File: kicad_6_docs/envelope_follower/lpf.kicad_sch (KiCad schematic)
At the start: 6 parts, among them U2 TL072

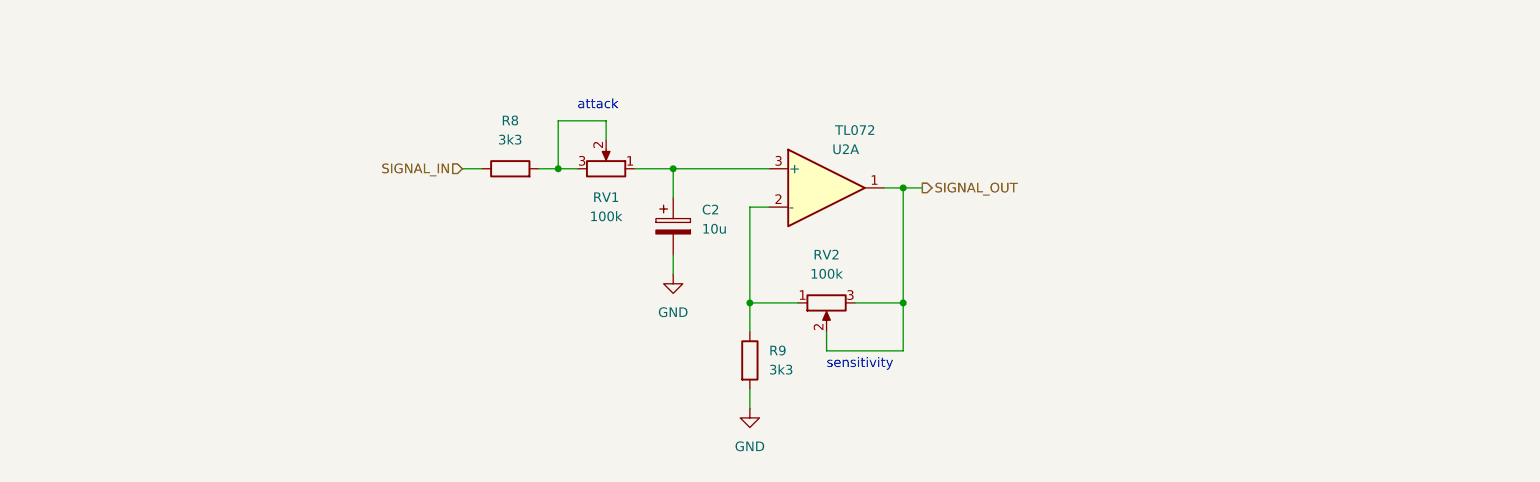
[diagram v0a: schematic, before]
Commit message: Env follower rev 0 and outputs
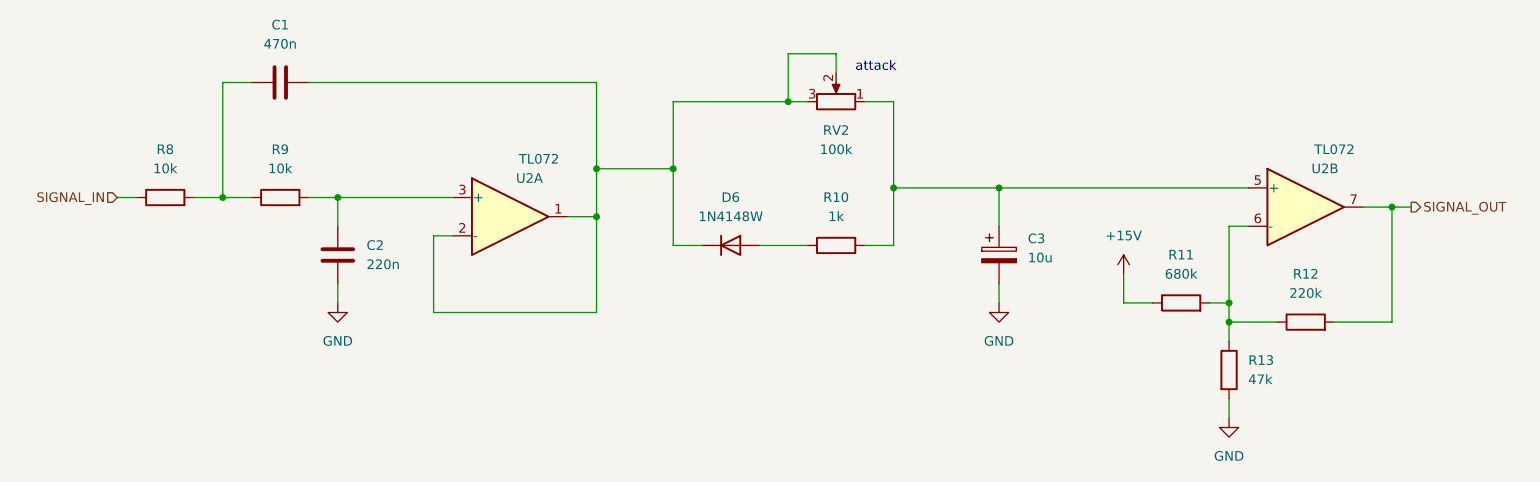
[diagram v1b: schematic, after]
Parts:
- removed C2: 10u, Capacitor_THT:CP_Radial_D6.3mm_P2.50mm, symbol Device:C_Polarized
- removed RV1: 100k, Potentiometer_THT:Potentiometer_Alpha_RD901F-40-00D_Single_Vertical, symbol Device:R_Potentiometer
- added C1: 470n, Capacitor_THT:C_Rect_L7.0mm_W3.5mm_P5.00mm, symbol Device:C
- added C2: 220n, Capacitor_THT:C_Rect_L7.0mm_W3.5mm_P5.00mm, symbol Device:C
- added C3: 10u, Capacitor_THT:CP_Radial_D6.3mm_P2.50mm, symbol Device:C_Polarized
- added D6: 1N4148W, Diode_SMD:D_SOD-123, symbol Diode:1N4148W
- added R10: 1k, Resistor_SMD:R_0805_2012Metric, symbol Device:R
- added R11: 680k, Resistor_SMD:R_0805_2012Metric, symbol Device:R
- added R12: 220k, Resistor_SMD:R_0805_2012Metric, symbol Device:R
- added R13: 47k, Resistor_SMD:R_0805_2012Metric, symbol Device:R
- added unit 2 of U2
- R8, R9: value 3k3 -> 10k
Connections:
- net GND: now also C2.2, C3.2, R13.2; no longer R9.2
- net SIGNAL_OUT: now also R12.2, U2.7; no longer RV2.2, RV2.3, U2.1
- net at U2.3 (+): now also R9.2, C2.1
- net at R8.2: now also R9.1, C1.1
- new net: C1.2, D6.1 (K), RV2.2, RV2.3, U2.1, U2.2 (-)
- new net: C3.1, R10.2, RV2.1, U2.5 (+)
- new net: D6.2 (A), R10.1
- new net: R11.2, R12.1, R13.1, U2.6 (-)
- new net +15V: R11.1
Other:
- note removed: "sensitivity"
